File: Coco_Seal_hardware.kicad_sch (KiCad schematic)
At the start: 47 parts, among them J1 E220-900T22S(JP), Q1 FS8205A, Q3 Q_NMOS_GSD, SW1 SOS_Button, SW2 Common_Button, SW3 Reset_Button, U1 TPD2EUSB30A, U2 ESP32-C3-WROOM-02, U3 TP4056-42-ESOP8, U5 AP2112K-3.3, U6 DW01A, U7 SSD1306_OLED

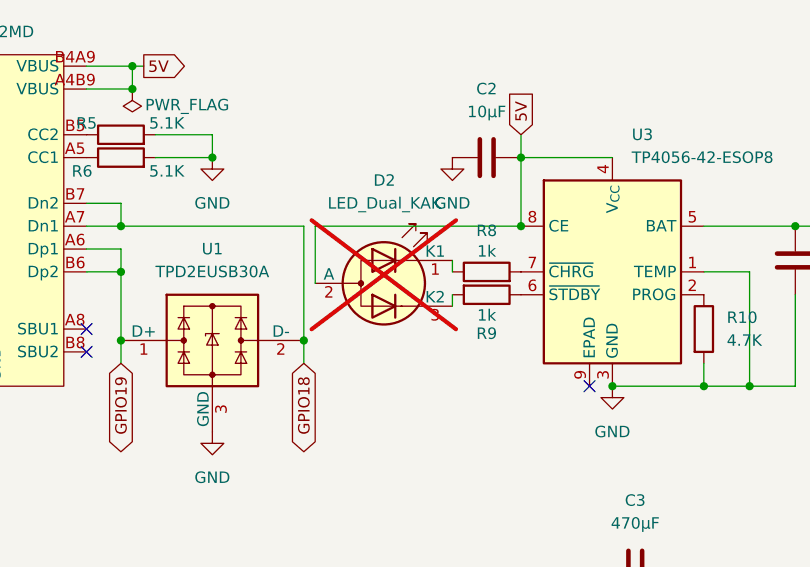
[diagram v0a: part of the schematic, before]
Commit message: 基板設計いったん完了
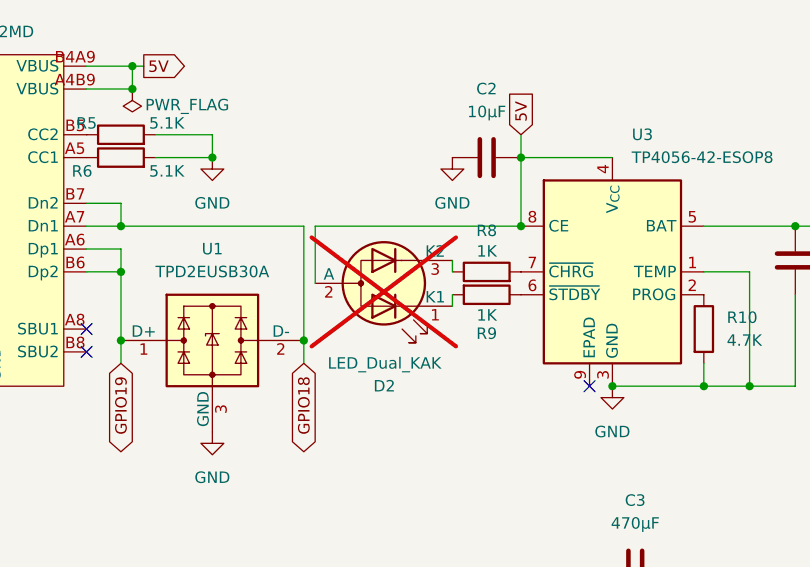
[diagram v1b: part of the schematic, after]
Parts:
- C1: LCSC Part (none) -> C15849
- C10, C3: LCSC Part (none) -> C3341
- C2, C4, C6, C8: LCSC Part (none) -> C13585
- C5, C7, C9: LCSC Part (none) -> C14663
- Q1: LCSC Part (none) -> C2830320
- Q3: LCSC Part (none) -> C20917
- R1, R2, R7: LCSC Part (none) -> C25804
- R10: LCSC Part (none) -> C23162
- R11, R12, R16: LCSC Part (none) -> C25803
- R13, R15: LCSC Part (none) -> C22775
- R14: LCSC Part (none) -> C21190
- R3, R4: LCSC Part (none) -> C23138
- R5, R6: LCSC Part (none) -> C23186
- R8, R9: value 1k -> 1K; LCSC Part (none) -> C21190
- SW2: LCSC Part (none) -> C557600
- SW3: LCSC Part (none) -> C97440
- U2: LCSC Part (none) -> C2934560
- U3: LCSC Part (none) -> C16581
- U5: LCSC Part (none) -> C23380830
- U6: LCSC Part (none) -> C351410
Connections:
- net at R9.2: now also D2.1 (K1); no longer D2.3 (K2)
- net at R8.1: now also D2.3 (K2); no longer D2.1 (K1)
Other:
- moved on the sheet: D2
